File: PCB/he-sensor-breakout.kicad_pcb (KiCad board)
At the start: 2 copper layers, 19.1 x 29.1 mm, 13 parts, among them J1 Conn_01x03, U1 SLSS49E

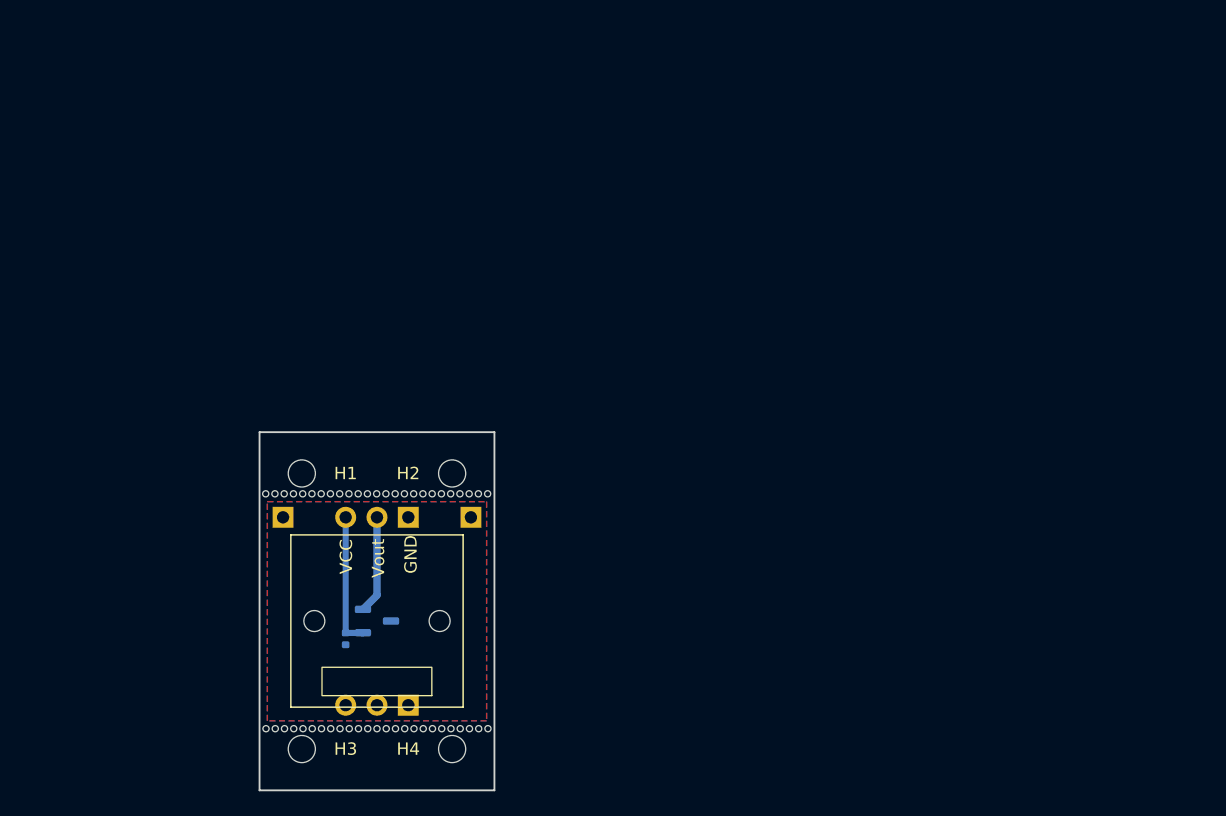
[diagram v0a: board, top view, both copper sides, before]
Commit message: makes sensor matrix
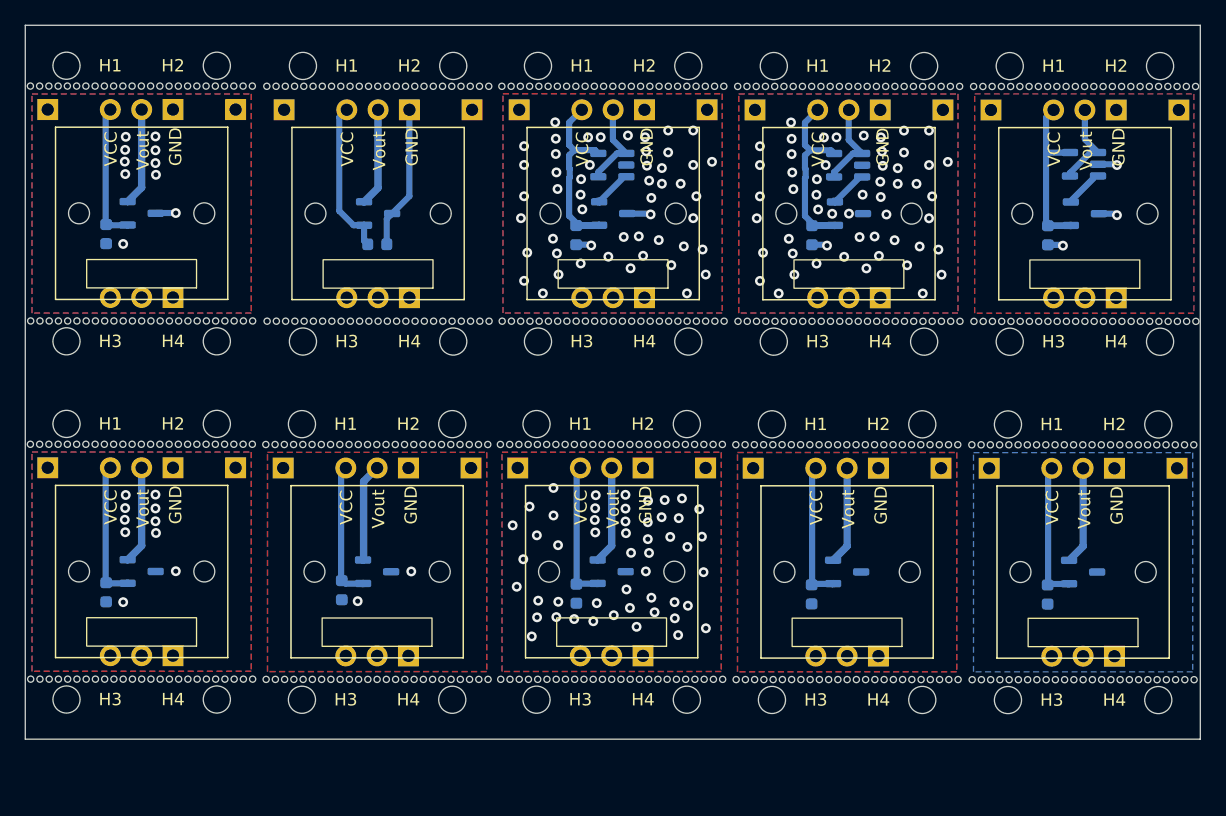
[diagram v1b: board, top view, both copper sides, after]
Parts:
- added C1: 100n, Capacitor_SMD:C_0603_1608Metric, B.Cu at (78.0, 69.4)
- added C1: 100n, Capacitor_SMD:C_0603_1608Metric, B.Cu at (116.2, 69.5)
- added C1: 100n, Capacitor_SMD:C_0603_1608Metric, B.Cu at (97.1, 98.3)
- added C1: 100n, Capacitor_SMD:C_0603_1608Metric, B.Cu at (154.4, 98.6)
- added C1: 100n, Capacitor_SMD:C_0603_1608Metric, B.Cu at (116.2, 98.6)
- added C1: 100n, Capacitor_SMD:C_0603_1608Metric, B.Cu at (135.3, 98.6)
- added C1: 100n, Capacitor_SMD:C_0603_1608Metric, B.Cu at (135.3, 69.5)
- added C1: 100n, Capacitor_SMD:C_0603_1608Metric, B.Cu at (100.0, 70.2)
- added C1: 100n, Capacitor_SMD:C_0603_1608Metric, B.Cu at (154.4, 69.5)
- added H1: MountingHole_2.2mm_M2, MountingHole:MountingHole_2.2mm_M2, F.Cu at (93.9, 84.8)
- added H1: MountingHole_2.2mm_M2, MountingHole:MountingHole_2.2mm_M2, F.Cu at (113.1, 55.8)
- added H1: MountingHole_2.2mm_M2, MountingHole:MountingHole_2.2mm_M2, F.Cu at (74.8, 55.8)
- added H1: MountingHole_2.2mm_M2, MountingHole:MountingHole_2.2mm_M2, F.Cu at (94.0, 55.8)
- added H1: MountingHole_2.2mm_M2, MountingHole:MountingHole_2.2mm_M2, F.Cu at (132.2, 55.8)
- added H1: MountingHole_2.2mm_M2, MountingHole:MountingHole_2.2mm_M2, F.Cu at (132.0, 84.8)
- added H1: MountingHole_2.2mm_M2, MountingHole:MountingHole_2.2mm_M2, F.Cu at (112.9, 84.8)
- added H1: MountingHole_2.2mm_M2, MountingHole:MountingHole_2.2mm_M2, F.Cu at (151.2, 84.9)
- added H1: MountingHole_2.2mm_M2, MountingHole:MountingHole_2.2mm_M2, F.Cu at (151.3, 55.8)
- added H2: MountingHole_2.2mm_M2, MountingHole:MountingHole_2.2mm_M2, F.Cu at (125.2, 55.8)
- added H2: MountingHole_2.2mm_M2, MountingHole:MountingHole_2.2mm_M2, F.Cu at (87.0, 55.8)
- added H2: MountingHole_2.2mm_M2, MountingHole:MountingHole_2.2mm_M2, F.Cu at (106.1, 84.8)
- added H2: MountingHole_2.2mm_M2, MountingHole:MountingHole_2.2mm_M2, F.Cu at (144.4, 55.8)
- added H2: MountingHole_2.2mm_M2, MountingHole:MountingHole_2.2mm_M2, F.Cu at (163.5, 55.8)
- added H2: MountingHole_2.2mm_M2, MountingHole:MountingHole_2.2mm_M2, F.Cu at (163.4, 84.9)
- added H2: MountingHole_2.2mm_M2, MountingHole:MountingHole_2.2mm_M2, F.Cu at (125.1, 84.8)
- added H2: MountingHole_2.2mm_M2, MountingHole:MountingHole_2.2mm_M2, F.Cu at (106.2, 55.8)
- added H2: MountingHole_2.2mm_M2, MountingHole:MountingHole_2.2mm_M2, F.Cu at (144.2, 84.8)
- added H3: MountingHole_2.2mm_M2, MountingHole:MountingHole_2.2mm_M2, F.Cu at (151.3, 78.1)
- added H3: MountingHole_2.2mm_M2, MountingHole:MountingHole_2.2mm_M2, F.Cu at (151.2, 107.2)
- added H3: MountingHole_2.2mm_M2, MountingHole:MountingHole_2.2mm_M2, F.Cu at (132.2, 78.1)
- added H3: MountingHole_2.2mm_M2, MountingHole:MountingHole_2.2mm_M2, F.Cu at (132.0, 107.2)
- added H3: MountingHole_2.2mm_M2, MountingHole:MountingHole_2.2mm_M2, F.Cu at (113.1, 78.1)
- added H3: MountingHole_2.2mm_M2, MountingHole:MountingHole_2.2mm_M2, F.Cu at (94.0, 78.1)
- added H3: MountingHole_2.2mm_M2, MountingHole:MountingHole_2.2mm_M2, F.Cu at (112.9, 107.2)
- added H3: MountingHole_2.2mm_M2, MountingHole:MountingHole_2.2mm_M2, F.Cu at (93.9, 107.2)
- added H3: MountingHole_2.2mm_M2, MountingHole:MountingHole_2.2mm_M2, F.Cu at (74.8, 78.1)
- added H4: MountingHole_2.2mm_M2, MountingHole:MountingHole_2.2mm_M2, F.Cu at (87.0, 78.1)
- added H4: MountingHole_2.2mm_M2, MountingHole:MountingHole_2.2mm_M2, F.Cu at (106.2, 78.1)
- added H4: MountingHole_2.2mm_M2, MountingHole:MountingHole_2.2mm_M2, F.Cu at (125.1, 107.2)
- added H4: MountingHole_2.2mm_M2, MountingHole:MountingHole_2.2mm_M2, F.Cu at (106.1, 107.2)
- added H4: MountingHole_2.2mm_M2, MountingHole:MountingHole_2.2mm_M2, F.Cu at (144.4, 78.1)
- added H4: MountingHole_2.2mm_M2, MountingHole:MountingHole_2.2mm_M2, F.Cu at (163.4, 107.2)
- added H4: MountingHole_2.2mm_M2, MountingHole:MountingHole_2.2mm_M2, F.Cu at (125.2, 78.1)
- added H4: MountingHole_2.2mm_M2, MountingHole:MountingHole_2.2mm_M2, F.Cu at (144.2, 107.2)
- added H4: MountingHole_2.2mm_M2, MountingHole:MountingHole_2.2mm_M2, F.Cu at (163.5, 78.1)
- added J1: Conn_01x03, Connector_PinHeader_2.54mm:PinHeader_1x03_P2.54mm_Vertical, B.Cu at (102.5, 88.4)
- added J1: Conn_01x03, Connector_PinHeader_2.54mm:PinHeader_1x03_P2.54mm_Vertical, B.Cu at (121.6, 88.4)
- added J1: Conn_01x03, Connector_PinHeader_2.54mm:PinHeader_1x03_P2.54mm_Vertical, B.Cu at (140.8, 59.3)
- added J1: Conn_01x03, Connector_PinHeader_2.54mm:PinHeader_1x03_P2.54mm_Vertical, B.Cu at (159.8, 88.4)
- added J1: Conn_01x03, Connector_PinHeader_2.54mm:PinHeader_1x03_P2.54mm_Vertical, B.Cu at (102.6, 59.3)
- added J1: Conn_01x03, Connector_PinHeader_2.54mm:PinHeader_1x03_P2.54mm_Vertical, B.Cu at (121.7, 59.3)
- added J1: Conn_01x03, Connector_PinHeader_2.54mm:PinHeader_1x03_P2.54mm_Vertical, B.Cu at (83.5, 59.3)
- added J1: Conn_01x03, Connector_PinHeader_2.54mm:PinHeader_1x03_P2.54mm_Vertical, B.Cu at (140.7, 88.4)
- added J1: Conn_01x03, Connector_PinHeader_2.54mm:PinHeader_1x03_P2.54mm_Vertical, B.Cu at (160.0, 59.3)
- added MOUSE1: mouse-bite-19mm, Panelization:mouse-bite-19mm, F.Cu at (100.0, 86.5)
- added MOUSE1: mouse-bite-19mm, Panelization:mouse-bite-19mm, F.Cu at (119.0, 86.5)
- added MOUSE1: mouse-bite-19mm, Panelization:mouse-bite-19mm, F.Cu at (119.1, 57.4)
- added MOUSE1: mouse-bite-19mm, Panelization:mouse-bite-19mm, F.Cu at (138.3, 57.4)
- added MOUSE1: mouse-bite-19mm, Panelization:mouse-bite-19mm, F.Cu at (100.1, 57.4)
- added MOUSE1: mouse-bite-19mm, Panelization:mouse-bite-19mm, F.Cu at (157.2, 86.5)
- added MOUSE1: mouse-bite-19mm, Panelization:mouse-bite-19mm, F.Cu at (157.4, 57.4)
- added MOUSE1: mouse-bite-19mm, Panelization:mouse-bite-19mm, F.Cu at (80.9, 57.4)
- added MOUSE1: mouse-bite-19mm, Panelization:mouse-bite-19mm, F.Cu at (138.1, 86.5)
- added MOUSE2: mouse-bite-19mm, Panelization:mouse-bite-19mm, F.Cu at (138.3, 76.5)
- added MOUSE2: mouse-bite-19mm, Panelization:mouse-bite-19mm, F.Cu at (80.9, 76.5)
- added MOUSE2: mouse-bite-19mm, Panelization:mouse-bite-19mm, F.Cu at (119.2, 76.5)
- added MOUSE2: mouse-bite-19mm, Panelization:mouse-bite-19mm, F.Cu at (157.4, 76.5)
- added MOUSE2: mouse-bite-19mm, Panelization:mouse-bite-19mm, F.Cu at (100.1, 76.5)
- added MOUSE2: mouse-bite-19mm, Panelization:mouse-bite-19mm, F.Cu at (100.0, 105.5)
- added MOUSE2: mouse-bite-19mm, Panelization:mouse-bite-19mm, F.Cu at (138.1, 105.5)
- added MOUSE2: mouse-bite-19mm, Panelization:mouse-bite-19mm, F.Cu at (119.0, 105.5)
- added MOUSE2: mouse-bite-19mm, Panelization:mouse-bite-19mm, F.Cu at (157.3, 105.6)
- added REF**: SOT-23-5, Package_TO_SOT_SMD:SOT-23-5, B.Cu at (119.1, 63.8)
- added REF**: SOT-23-5, Package_TO_SOT_SMD:SOT-23-5, B.Cu at (157.3, 63.7)
- added REF**: SOT-23-5, Package_TO_SOT_SMD:SOT-23-5, B.Cu at (138.2, 63.8)
- added STB1: PinHeader_1x01_P2.54mm_Vertical, Connector_PinHeader_2.54mm:PinHeader_1x01_P2.54mm_Vertical, B.Cu at (130.7, 59.3)
- added STB1: PinHeader_1x01_P2.54mm_Vertical, Connector_PinHeader_2.54mm:PinHeader_1x01_P2.54mm_Vertical, B.Cu at (111.5, 59.3)
- added STB1: PinHeader_1x01_P2.54mm_Vertical, Connector_PinHeader_2.54mm:PinHeader_1x01_P2.54mm_Vertical, B.Cu at (149.8, 59.3)
- added STB1: PinHeader_1x01_P2.54mm_Vertical, Connector_PinHeader_2.54mm:PinHeader_1x01_P2.54mm_Vertical, B.Cu at (92.4, 88.4)
- added STB1: PinHeader_1x01_P2.54mm_Vertical, Connector_PinHeader_2.54mm:PinHeader_1x01_P2.54mm_Vertical, B.Cu at (111.4, 88.4)
- added STB1: PinHeader_1x01_P2.54mm_Vertical, Connector_PinHeader_2.54mm:PinHeader_1x01_P2.54mm_Vertical, B.Cu at (92.5, 59.3)
- added STB1: PinHeader_1x01_P2.54mm_Vertical, Connector_PinHeader_2.54mm:PinHeader_1x01_P2.54mm_Vertical, B.Cu at (130.5, 88.4)
- added STB1: PinHeader_1x01_P2.54mm_Vertical, Connector_PinHeader_2.54mm:PinHeader_1x01_P2.54mm_Vertical, B.Cu at (73.3, 59.3)
- added STB1: PinHeader_1x01_P2.54mm_Vertical, Connector_PinHeader_2.54mm:PinHeader_1x01_P2.54mm_Vertical, B.Cu at (149.7, 88.4)
- added STB2: PinHeader_1x01_P2.54mm_Vertical, Connector_PinHeader_2.54mm:PinHeader_1x01_P2.54mm_Vertical, B.Cu at (126.7, 88.4)
- added STB2: PinHeader_1x01_P2.54mm_Vertical, Connector_PinHeader_2.54mm:PinHeader_1x01_P2.54mm_Vertical, B.Cu at (88.5, 59.3)
- added STB2: PinHeader_1x01_P2.54mm_Vertical, Connector_PinHeader_2.54mm:PinHeader_1x01_P2.54mm_Vertical, B.Cu at (107.7, 59.3)
- added STB2: PinHeader_1x01_P2.54mm_Vertical, Connector_PinHeader_2.54mm:PinHeader_1x01_P2.54mm_Vertical, B.Cu at (165.0, 59.3)
- added STB2: PinHeader_1x01_P2.54mm_Vertical, Connector_PinHeader_2.54mm:PinHeader_1x01_P2.54mm_Vertical, B.Cu at (107.6, 88.4)
- added STB2: PinHeader_1x01_P2.54mm_Vertical, Connector_PinHeader_2.54mm:PinHeader_1x01_P2.54mm_Vertical, B.Cu at (164.9, 88.4)
- added STB2: PinHeader_1x01_P2.54mm_Vertical, Connector_PinHeader_2.54mm:PinHeader_1x01_P2.54mm_Vertical, B.Cu at (145.9, 59.3)
- added STB2: PinHeader_1x01_P2.54mm_Vertical, Connector_PinHeader_2.54mm:PinHeader_1x01_P2.54mm_Vertical, B.Cu at (145.7, 88.4)
- added STB2: PinHeader_1x01_P2.54mm_Vertical, Connector_PinHeader_2.54mm:PinHeader_1x01_P2.54mm_Vertical, B.Cu at (126.8, 59.3)
- added STB3: PinHeader_1x03_P2.54mm_Vertical, Connector_PinHeader_2.54mm:PinHeader_1x03_P2.54mm_Vertical, B.Cu at (83.5, 74.6)
- added STB3: PinHeader_1x03_P2.54mm_Vertical, Connector_PinHeader_2.54mm:PinHeader_1x03_P2.54mm_Vertical, B.Cu at (121.6, 103.6)
- added STB3: PinHeader_1x03_P2.54mm_Vertical, Connector_PinHeader_2.54mm:PinHeader_1x03_P2.54mm_Vertical, B.Cu at (159.8, 103.6)
- added STB3: PinHeader_1x03_P2.54mm_Vertical, Connector_PinHeader_2.54mm:PinHeader_1x03_P2.54mm_Vertical, B.Cu at (160.0, 74.6)
- added STB3: PinHeader_1x03_P2.54mm_Vertical, Connector_PinHeader_2.54mm:PinHeader_1x03_P2.54mm_Vertical, B.Cu at (102.5, 103.6)
- added STB3: PinHeader_1x03_P2.54mm_Vertical, Connector_PinHeader_2.54mm:PinHeader_1x03_P2.54mm_Vertical, B.Cu at (140.8, 74.6)
- added STB3: PinHeader_1x03_P2.54mm_Vertical, Connector_PinHeader_2.54mm:PinHeader_1x03_P2.54mm_Vertical, B.Cu at (102.6, 74.6)
- added STB3: PinHeader_1x03_P2.54mm_Vertical, Connector_PinHeader_2.54mm:PinHeader_1x03_P2.54mm_Vertical, B.Cu at (140.7, 103.6)
- added STB3: PinHeader_1x03_P2.54mm_Vertical, Connector_PinHeader_2.54mm:PinHeader_1x03_P2.54mm_Vertical, B.Cu at (121.7, 74.6)
- added SW: SW_Lekker_MX_1.00u_PCB, Button_Switch_Keyboard:SW_Lekker_MX_1.00u_PCB, F.Cu at (80.9, 67.7)
- added SW: SW_Lekker_MX_1.00u_PCB, Button_Switch_Keyboard:SW_Lekker_MX_1.00u_PCB, F.Cu at (119.0, 96.8)
- added SW: SW_Lekker_MX_1.00u_PCB, Button_Switch_Keyboard:SW_Lekker_MX_1.00u_PCB, F.Cu at (138.3, 67.8)
- added SW: SW_Lekker_MX_1.00u_PCB, Button_Switch_Keyboard:SW_Lekker_MX_1.00u_PCB, F.Cu at (138.1, 96.8)
- added SW: SW_Lekker_MX_1.00u_PCB, Button_Switch_Keyboard:SW_Lekker_MX_1.00u_PCB, F.Cu at (119.2, 67.7)
- added SW: SW_Lekker_MX_1.00u_PCB, Button_Switch_Keyboard:SW_Lekker_MX_1.00u_PCB, F.Cu at (100.1, 67.7)
- added SW: SW_Lekker_MX_1.00u_PCB, Button_Switch_Keyboard:SW_Lekker_MX_1.00u_PCB, F.Cu at (157.4, 67.8)
- added SW: SW_Lekker_MX_1.00u_PCB, Button_Switch_Keyboard:SW_Lekker_MX_1.00u_PCB, F.Cu at (157.3, 96.8)
- added SW: SW_Lekker_MX_1.00u_PCB, Button_Switch_Keyboard:SW_Lekker_MX_1.00u_PCB, F.Cu at (100.0, 96.8)
- added U1: SLSS49E, Package_TO_SOT_SMD:SOT-23-3, B.Cu at (119.2, 67.7)
- added U1: SLSS49E, Package_TO_SOT_SMD:SOT-23-3, B.Cu at (138.1, 96.8)
- added U1: SLSS49E, Package_TO_SOT_SMD:SOT-23-3, B.Cu at (80.9, 67.7)
- added U1: SLSS49E, Package_TO_SOT_SMD:SOT-23-3, B.Cu at (138.3, 67.8)
- added U1: SLSS49E, Package_TO_SOT_SMD:SOT-23-3, B.Cu at (157.3, 96.8)
- added U1: SLSS49E, Package_TO_SOT_SMD:SOT-23-3, B.Cu at (119.0, 96.8)
- added U1: SLSS49E, Package_TO_SOT_SMD:SOT-23-3, B.Cu at (100.1, 67.7)
- added U1: SLSS49E, Package_TO_SOT_SMD:SOT-23-3, B.Cu at (100.0, 96.8)
- added U1: SLSS49E, Package_TO_SOT_SMD:SOT-23-3, B.Cu at (157.4, 67.8)
- C1: footprint Capacitor_SMD:C_0402_1005Metric -> Capacitor_SMD:C_0603_1608Metric
- moved C1 19.8 mm to (78.0, 98.5)
- moved MOUSE2 19.5 mm to (80.9, 105.5)
- moved STB3 19.5 mm to (83.5, 103.6)
- moved H2 19.5 mm to (87.0, 84.8)
- moved H4 19.5 mm to (87.0, 107.2)
- moved J1 19.5 mm to (83.5, 88.4)
- moved STB2 19.5 mm to (88.5, 88.4)
- moved SW 19.5 mm to (80.9, 96.8)
- moved U1 19.5 mm to (80.9, 96.8)
- moved H1 19.5 mm to (74.8, 84.8)
- moved H3 19.5 mm to (74.8, 107.2)
- moved MOUSE1 19.5 mm to (80.9, 86.5)
- moved STB1 19.5 mm to (73.3, 88.4)
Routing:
- net VCC: track 10.8 -> 125.2 mm
- net /Vout: track 7.96 -> 77.4 mm
- net GND: track 0.00 -> 22.1 mm, vias 0 -> 180
- net Sout: track 0.00 -> 9.23 mm
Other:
- board size 19.1 x 29.1 mm -> 95.3 x 57.9 mm
